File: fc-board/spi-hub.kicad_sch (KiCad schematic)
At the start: 22 parts, among them J15 BCS-110-L-D-TE, U10 LTC2983ILX-PBF

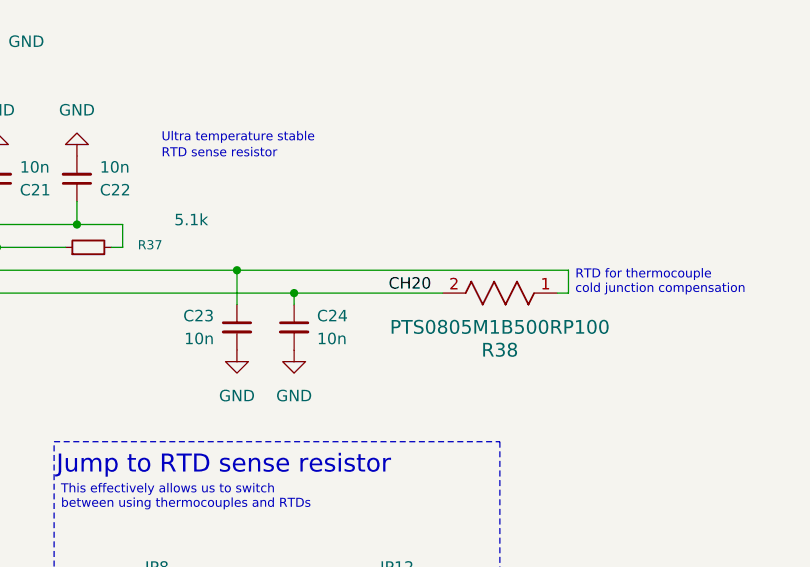
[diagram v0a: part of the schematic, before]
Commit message: some updates
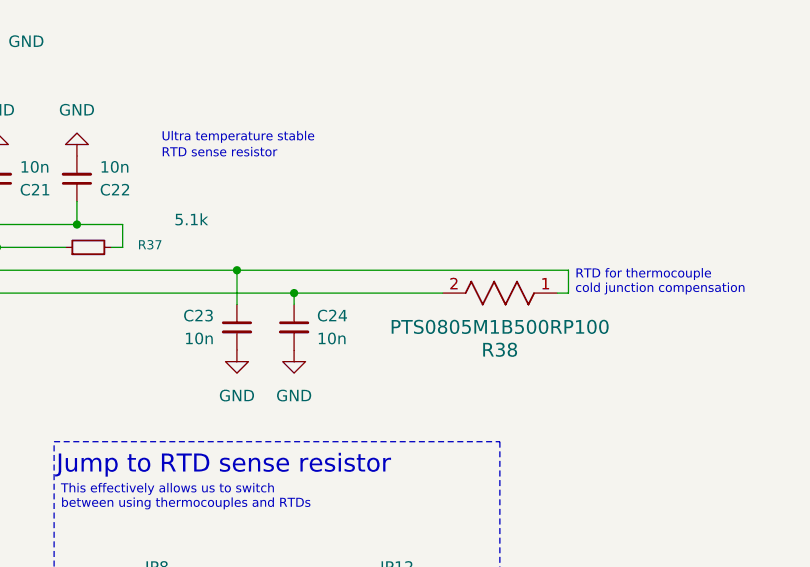
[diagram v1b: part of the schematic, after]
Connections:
- net CH17: no longer C22.1, J15.20, JP10.2 (B), JP11.2 (B), JP12.2 (B), JP13.2 (B), JP14.2 (B), JP15.2 (B), JP8.2 (B), JP9.2 (B), R37.2, U10.35 (CH20)
- new net CH20: C22.1, J15.20, JP10.2 (B), JP11.2 (B), JP12.2 (B), JP13.2 (B), JP14.2 (B), JP15.2 (B), JP8.2 (B), JP9.2 (B), R37.2, U10.35 (CH20)
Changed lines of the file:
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@@
-		)
-	)
-	(label "CH20"
-		(at 163.83 69.85 180)
-		(effects
-			(font
-				(size 1.27 1.27)
-			)
-			(justify right bottom)
 		)
 	)
